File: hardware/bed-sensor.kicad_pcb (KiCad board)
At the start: 2 copper layers, 40 parts, among them J1 USB_B_Mini, J2 Conn_ARM_JTAG_SWD_10, J3 DM3AT-SF-PEJM5, SW1 SW_Push, U1 MCP73831-2-OT, U2 TLV70218_SOT23-5, U3 AP2112K-3.3, U4 MDBT50Q-1M, U6 ICM-20948, U7 BMP280

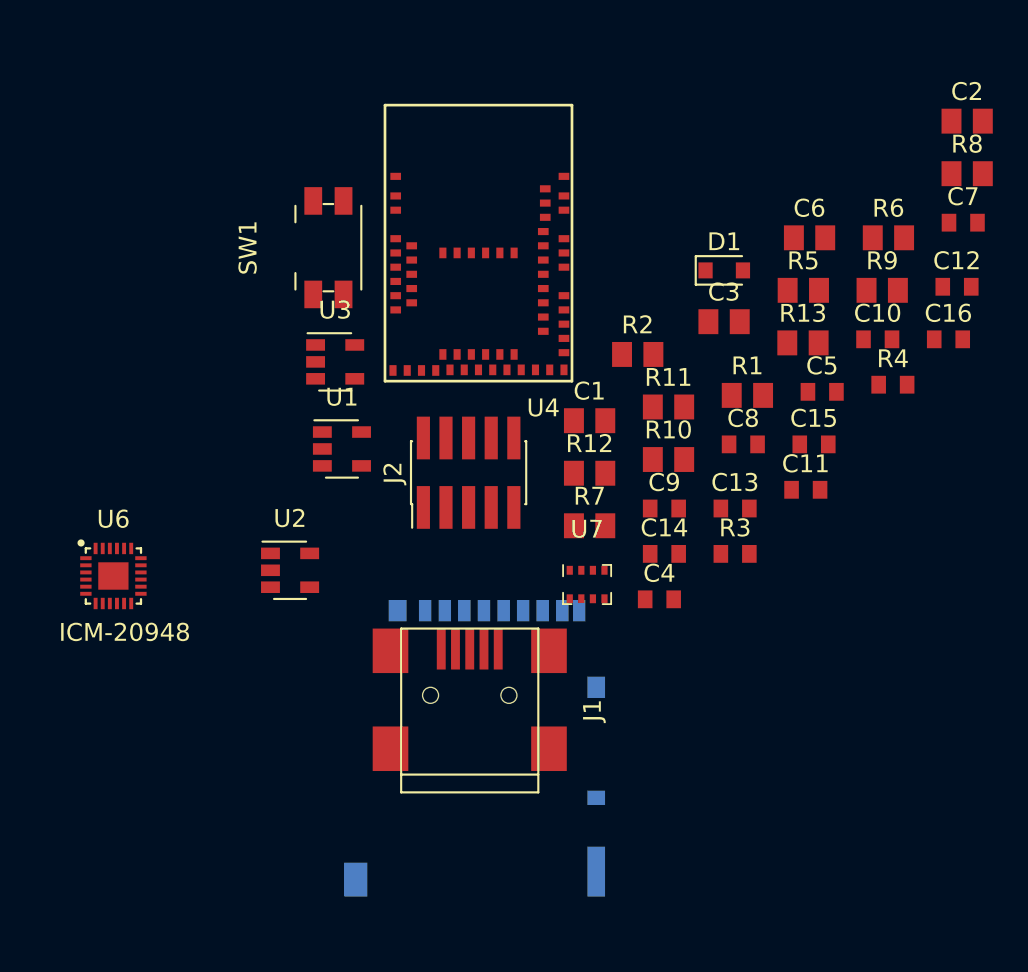
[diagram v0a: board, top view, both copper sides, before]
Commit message: started building board
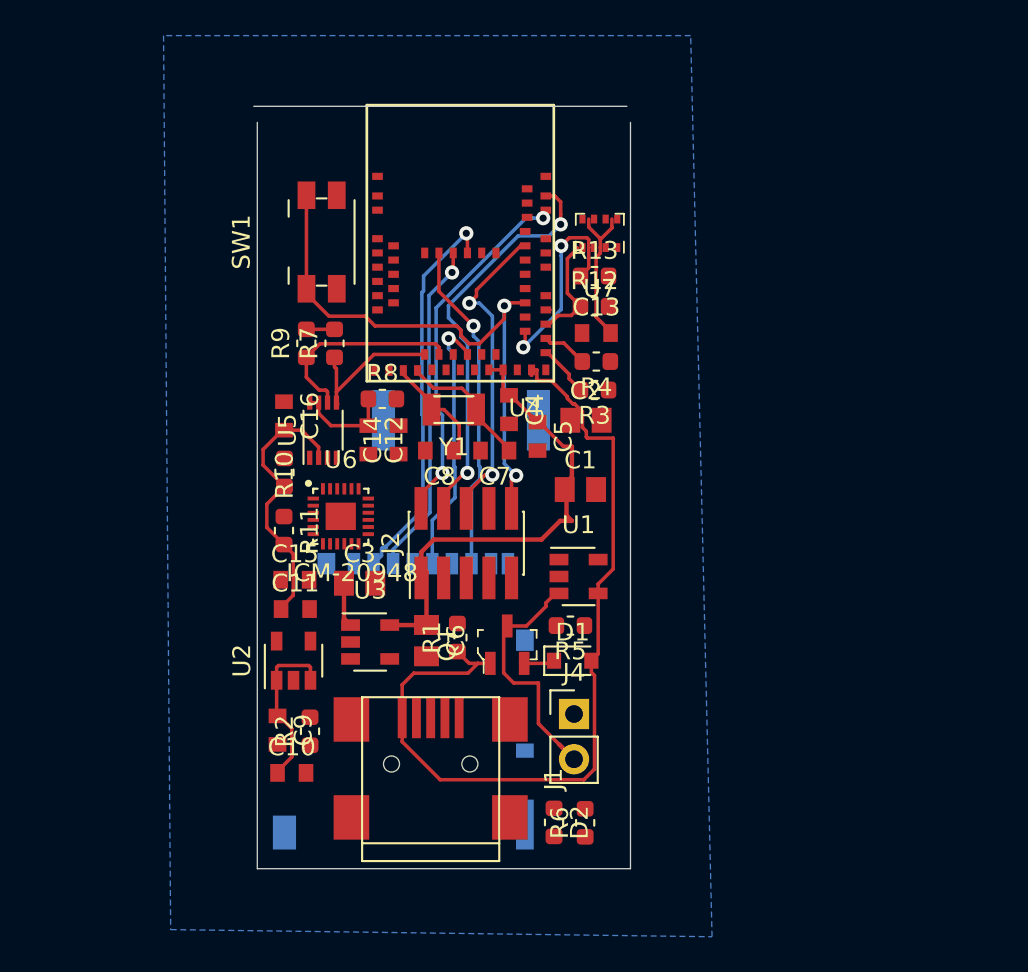
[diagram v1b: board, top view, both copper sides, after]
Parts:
- added BZ1: Buzzer, Buzzer_Beeper:Buzzer_Murata_PKMCS0909E4000-R1, B.Cu at (125.3, -31.9)
- added D2: LED, Capacitor_SMD:C_0603_1608Metric, F.Cu at (130.5, -9.32)
- added J4: Conn_01x02, Connector_PinHeader_2.54mm:PinHeader_1x02_P2.54mm_Vertical, F.Cu at (131.7, -15.4)
- added Q1: Q_PMOS_GSD, digikey-footprints:SOT-23-3, F.Cu at (127.9, -19.3)
- added U5: PCA9306, Package_SO:VSSOP-8_2.3x2mm_P0.5mm, F.Cu at (117.6, -31.3)
- added Y1: 32.768, OPL_Crystal_Oscillator:X2-SMD-3.2X1.5X0.55MM, F.Cu at (124.9, -32.5)
- R1, R10, R11, R12, R13, R2, R5, R6, R7, R8, R9: footprint Resistor_SMD:R_0805_2012Metric -> Fuse:Fuse_0603_1608Metric
- R3, R4: footprint Resistor_SMD:R_0603_1608Metric -> Fuse:Fuse_0603_1608Metric
- moved C10 40.9 mm to (115.8, -12.1)
- moved C16 37.6 mm to (115.4, -32.1), turned to 270 degrees
- moved R6 37.0 mm to (132.3, -9.30), turned to 90 degrees
- moved R8 35.2 mm to (120.9, -33.1)
- moved C12 34.2 mm to (120.1, -30.8), turned to 270 degrees
- moved R9 32.5 mm to (116.6, -36.2), turned to 90 degrees
- moved C6 31.2 mm to (123.4, -19.5), turned to 270 degrees
- moved C15 30.1 mm to (116.0, -22.9)
- moved C11 29.4 mm to (116.0, -21.3)
- moved C7 29.3 mm to (127.2, -30.2), turned to 180 degrees
- moved R2 28.0 mm to (116.8, -14.4), turned to 90 degrees
- moved C2 27.2 mm to (132.3, -31.9)
- moved C3 25.2 mm to (119.6, -22.7)
- moved C9 25.0 mm to (115.0, -14.5), turned to 270 degrees
- moved D1 23.5 mm to (131.6, -18.4)
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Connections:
- J1 pad 4: Net-(J1-Pad4) -> (no net)
- J2 pad 8: Net-(J2-Pad8) -> (no net)
- J3 pad 1: Net-(J3-Pad1) -> (no net)
- J3 pad 8: Net-(J3-Pad8) -> (no net)
- J3 pad SWA: Net-(J3-PadSWA) -> (no net)
- J3 pad SWB: Net-(J3-PadSWB) -> (no net)
- U2 pad 4: Net-(U2-Pad4) -> (no net)
- U3 pad 4: Net-(U3-Pad4) -> (no net)
- U4 pad 1: Net-(U4-Pad1) -> GND
- U4 pad 10: Net-(U4-Pad10) -> (no net)
- U4 pad 11: Net-(U4-Pad11) -> (no net)
- U4 pad 12: Net-(U4-Pad12) -> (no net)
- U4 pad 13: Net-(U4-Pad13) -> (no net)
- U4 pad 14: Net-(U4-Pad14) -> (no net)
- U4 pad 15: Net-(U4-Pad15) -> GND
- U4 pad 16: Net-(U4-Pad16) -> (no net)
- U4 pad 19: Net-(U4-Pad19) -> SCL_MPU
- U4 pad 20: Net-(U4-Pad20) -> (no net)
- U4 pad 21: Net-(U4-Pad21) -> SDA_MPU
- U4 pad 22: SCL_MPU -> (no net)
- U4 pad 23: Net-(U4-Pad23) -> (no net)
- U4 pad 24: SDA_MPU -> (no net)
- U4 pad 26: Net-(U4-Pad26) -> (no net)
- U4 pad 27: Net-(U4-Pad27) -> (no net)
- U4 pad 29: Net-(U4-Pad29) -> (no net)
- U4 pad 3: Net-(U4-Pad3) -> (no net)
- U4 pad 31: Net-(U4-Pad31) -> (no net)
- U4 pad 33: Net-(U4-Pad15) -> GND
- U4 pad 38: Net-(U4-Pad38) -> (no net)
- U4 pad 4: Net-(U4-Pad4) -> (no net)
- U4 pad 41: Net-(U4-Pad41) -> (no net)
- U4 pad 42: Net-(U4-Pad42) -> (no net)
- U4 pad 43: Net-(U4-Pad43) -> (no net)
- U4 pad 44: Net-(U4-Pad44) -> (no net)
- U4 pad 45: Net-(U4-Pad45) -> (no net)
- U4 pad 46: Net-(U4-Pad46) -> (no net)
- U4 pad 48: Net-(U4-Pad48) -> (no net)
- U4 pad 5: Net-(U4-Pad5) -> (no net)
- U4 pad 50: Net-(U4-Pad50) -> (no net)
- U4 pad 52: Net-(U4-Pad52) -> (no net)
- U4 pad 54: Net-(U4-Pad54) -> (no net)
- U4 pad 56: Net-(U4-Pad56) -> (no net)
- U4 pad 6: Net-(U4-Pad6) -> (no net)
- U4 pad 60: Net-(U4-Pad60) -> (no net)
- U4 pad 61: Net-(U4-Pad61) -> (no net)
- U4 pad 7: Net-(U4-Pad7) -> (no net)
- U4 pad 8: Net-(U4-Pad8) -> (no net)
- U4 pad 9: Net-(U4-Pad9) -> (no net)
- U6 pad 12: Net-(U6-Pad12) -> (no net)
- U6 pad 19: Net-(U6-Pad19) -> (no net)
- U6 pad 21: Net-(U6-Pad21) -> (no net)
- U6 pad 7: Net-(U6-Pad7) -> (no net)
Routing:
- net VBUS: track 0.00 -> 48.0 mm
- net +3V3: track 0.00 -> 46.5 mm
- net RESET: track 0.00 -> 32.5 mm, vias 0 -> 2
- net SWCLK: track 0.00 -> 23.2 mm, vias 0 -> 2
- net SD_CS: track 0.00 -> 22.0 mm, vias 0 -> 1
- net SWDIO: track 0.00 -> 20.8 mm, vias 0 -> 2
- net SD_MOSI: track 0.00 -> 18.9 mm, vias 0 -> 1
- net SD_MISO: track 0.00 -> 18.6 mm, vias 0 -> 1
- net SWO: track 0.00 -> 18.0 mm, vias 0 -> 2
- net +1V8: track 0.00 -> 15.3 mm
- net +BATT: track 0.00 -> 15.1 mm
- net SD_SCK: track 0.00 -> 14.8 mm, vias 0 -> 1
- net BMP_SDA: track 0.00 -> 11.9 mm, vias 0 -> 2
- net SDA_MPU: track 0.00 -> 11.5 mm
- net SCL_MPU: track 0.00 -> 8.53 mm
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- added copper zone on B.Cu, net GND
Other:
- board outline added: 21.2 x 42.8 mm
- net class Default: trace_width 0.25 -> 0.2
